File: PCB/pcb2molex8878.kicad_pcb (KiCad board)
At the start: 2 copper layers, 16 x 38.2 mm, 1 part

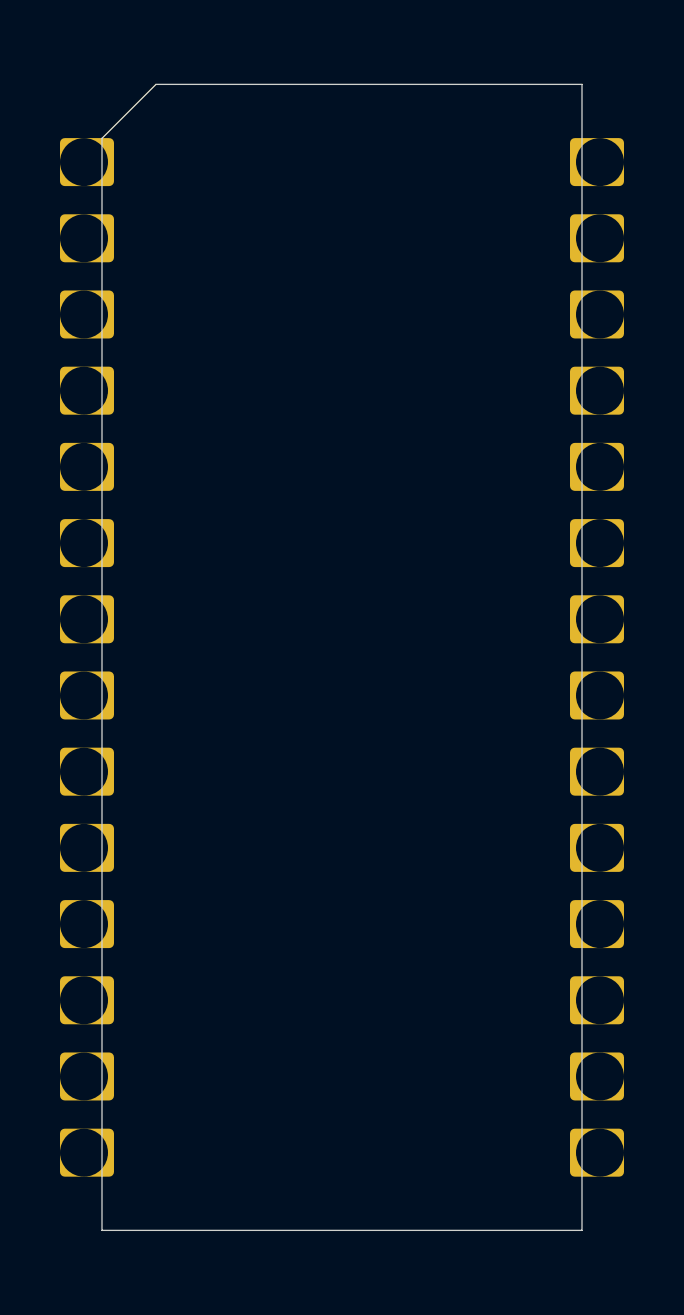
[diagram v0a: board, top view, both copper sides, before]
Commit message: finish 'max' variant
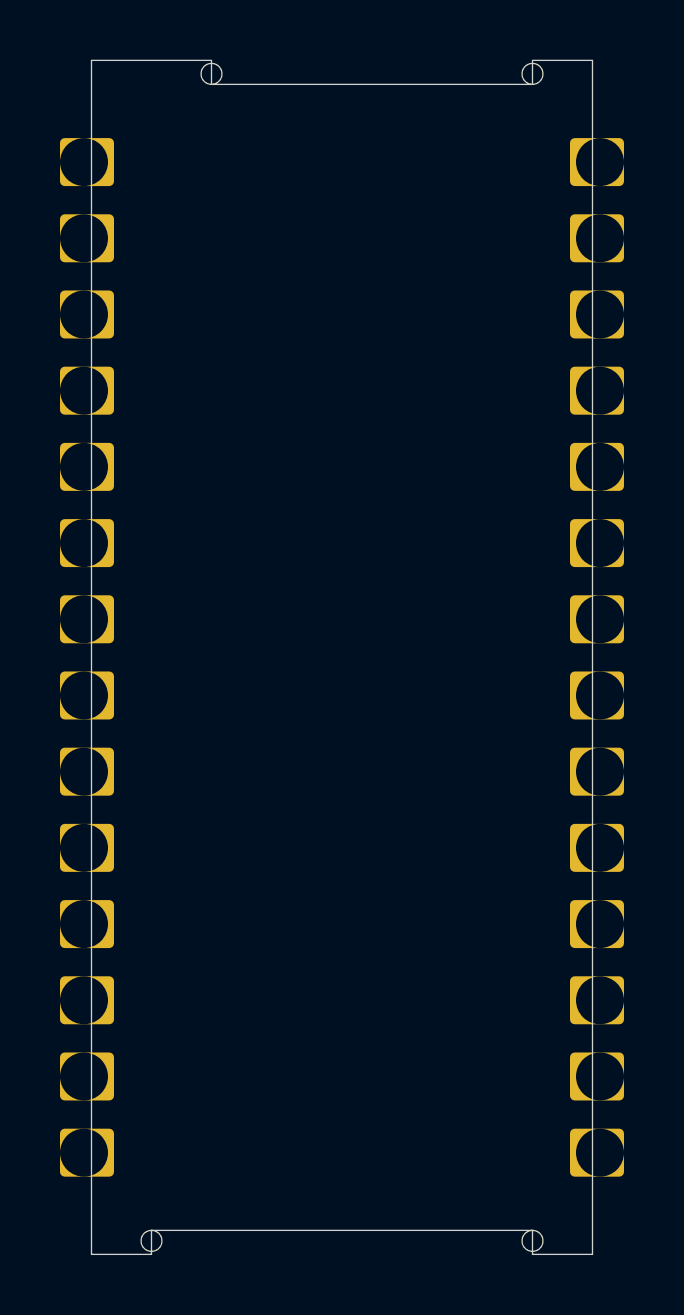
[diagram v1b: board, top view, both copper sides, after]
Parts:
- added REF**: MountingHole_2.2mm_M2, Mounting_Holes:MountingHole_2.2mm_M2, F.Cu at (140.9, 118.6)
- added REF**: MountingHole_2.2mm_M2, Mounting_Holes:MountingHole_2.2mm_M2, F.Cu at (153.6, 118.6)
- added REF**: MountingHole_2.2mm_M2, Mounting_Holes:MountingHole_2.2mm_M2, F.Cu at (153.6, 79.7)
- added REF**: MountingHole_2.2mm_M2, Mounting_Holes:MountingHole_2.2mm_M2, F.Cu at (142.9, 79.7)
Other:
- board size 16 x 38.2 mm -> 16.7 x 39.8 mm
- rule via_min_size: 0.508 -> 0.254
- board text added: "edge of hole to edge of hole"

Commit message: fix fitment clearance around prong detents. improve pcb model
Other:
- board text added: "partial mill radius fillet"
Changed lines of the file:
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@@
   (general
     (thickness 1.6)
-    (drawings 26)
+    (drawings 35)
     (tracks 0)
     (zones 0)
@@
     (38 B.Mask user)
     (39 F.Mask user)
-    (40 Dwgs.User user hide)
+    (40 Dwgs.User user)
     (41 Cmts.User user hide)
     (42 Eco1.User user hide)
@@
     (pad "" np_thru_hole circle (at 0 0) (size 0.7 0.7) (drill 0.7) (layers *.Cu *.Mask))
   )
+  (gr_line (start 141.2184 118.237) (end 141.4184 118.037) (layer Dwgs.User) (width 0.0127))
+  (gr_line (start 141.2184 118.237) (end 141.0184 118.037) (layer Dwgs.User) (width 0.0127))
+  (gr_text "partial mill radius fillet" (at 144.3184 117.287) (layer Dwgs.User)
+    (effects (font (size 0.4572 0.4572) (thickness 0.0127)))
+  )
+  (gr_line (start 141.2184 118.237) (end 141.2184 117.687) (layer Dwgs.User) (width 0.0127))
+  (gr_poly (pts (xy 140.8684 118.286575) (xy 141.7284 118.286855) (xy 141.59738 118.29796) (xy 141.52118 118.3132) (xy 141.47546 118.3259) (xy 141.41704 118.34622) (xy 141.37386 118.364) (xy 141.3383 118.38178) (xy 141.30782 118.39702) (xy 141.2875 118.40972) (xy 141.27226 118.41988) (xy 141.23924 118.4402) (xy 141.20876 118.46306) (xy 141.183724 118.481284) (xy 141.15796 118.4402) (xy 141.13256 118.40718) (xy 141.10208 118.3767) (xy 141.0716 118.3513) (xy 141.02842 118.3259) (xy 140.9954 118.31066) (xy 140.96492 118.3005) (xy 140.92936 118.29288) (xy 140.90904 118.29034)) (layer Dwgs.User) (width 0.001))
+  (dimension 0.860058 (width 0.0127) (layer Dwgs.User)
+    (gr_text "   0.86 mill radius" (at 141.314303 120.519679 0.7) (layer Dwgs.User)
+      (effects (font (size 0.4572 0.4572) (thickness 0.0127)) (justify left))
+    )
+    (feature1 (pts (xy 141.7284 119.147) (xy 141.74551 120.618493)))
+    (feature2 (pts (xy 140.8684 119.157) (xy 140.88551 120.628493)))
+    (crossbar (pts (xy 140.878692 120.042112) (xy 141.738692 120.032112)))
+    (arrow1a (pts (xy 141.738692 120.032112) (xy 140.619083 120.631591)))
+    (arrow1b (pts (xy 141.738692 120.032112) (xy 140.605446 119.458829)))
+    (arrow2a (pts (xy 140.878692 120.042112) (xy 142.011938 120.615395)))
+    (arrow2b (pts (xy 140.878692 120.042112) (xy 141.998301 119.442633)))
+  )
+  (gr_arc (start 141.7284 119.147) (end 141.7284 118.286855) (angle -39.28940686) (layer Dwgs.User) (width 0.0127))
+  (gr_arc (start 140.8684 118.637) (end 141.183359 118.483381) (angle -63.99944981) (layer Dwgs.User) (width 0.0127))
+  (gr_line (start 140.8684 118.287) (end 141.7284 118.286855) (layer Dwgs.User) (width 0.0127))
   (gr_text "edge of hole to edge of hole" (at 147.2184 122.887) (layer Dwgs.User)
     (effects (font (size 0.4572 0.4572) (thickness 0.0127)))
@@
   (gr_line (start 138.8684 79.287) (end 155.5684 119.087) (layer Dwgs.User) (width 0.0127))
   (gr_arc (start 152.7084 79.227) (end 152.7084 80.087) (angle -86.0090869) (layer Dwgs.User) (width 0.0127))
-  (gr_arc (start 143.7284 79.227) (end 142.868401 79.286999) (angle -86.0090869) (layer Dwgs.User) (width 0.0127))
-  (gr_arc (start 141.726315 119.146855) (end 141.726315 118.286855) (angle -86.0090869) (layer Dwgs.User) (width 0.0127))
+  (gr_arc (start 143.728401 79.224911) (end 142.868402 79.28491) (angle -86.0090869) (layer Dwgs.User) (width 0.0127))
+  (gr_arc (start 141.7284 119.146855) (end 141.7284 118.286855) (angle -86.0090869) (layer Dwgs.User) (width 0.0127))
   (gr_arc (start 152.708399 119.149089) (end 153.568398 119.08909) (angle -86.0090869) (layer Dwgs.User) (width 0.0127))
   (gr_line (start 153.5684 80.087) (end 153.5684 79.287) (layer Edge.Cuts) (width 0.0254))
